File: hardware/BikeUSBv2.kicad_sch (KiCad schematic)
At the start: 55 parts, among them J1 TYPE-C-31-M-16, J2 JST S2B-EH(LF)(SN), Q1 2SB772SQ, SW1 1TS002E-2500-2501-CT, SW2 1TS002E-2500-2501-CT, U1 TPS63070, U2 ATtiny1616-M, U3 FUSB302B10MPX, U4 HT7550, U5 TL431AIDBZR

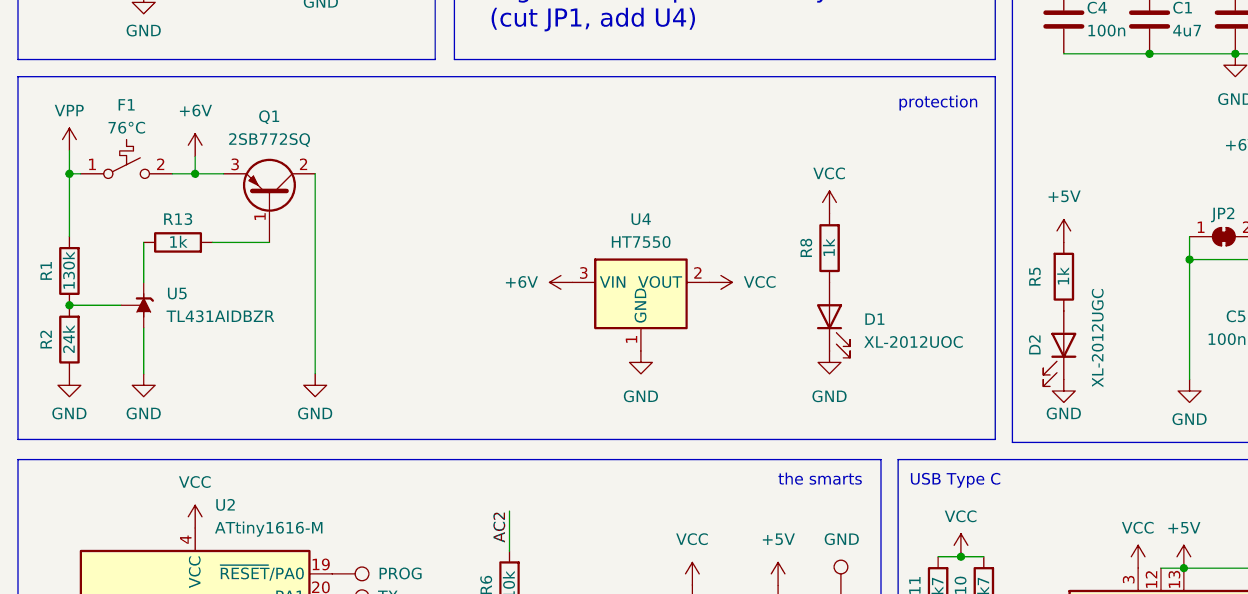
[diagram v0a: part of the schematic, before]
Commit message: idk
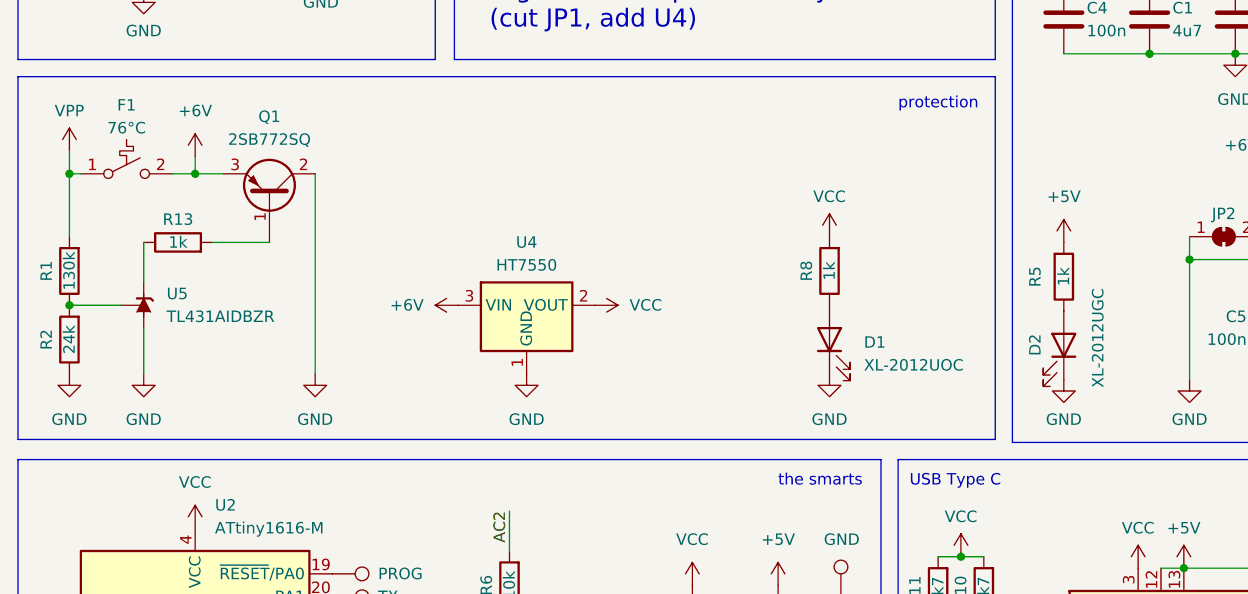
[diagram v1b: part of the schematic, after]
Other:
- moved on the sheet: D1, R8, U4
